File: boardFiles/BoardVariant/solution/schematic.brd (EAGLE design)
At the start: 75.9 x 38.1 mm, 45 parts, among them IC1 MSP430F1491, IC3 CP2102, U1 TPS62122_DRV_6

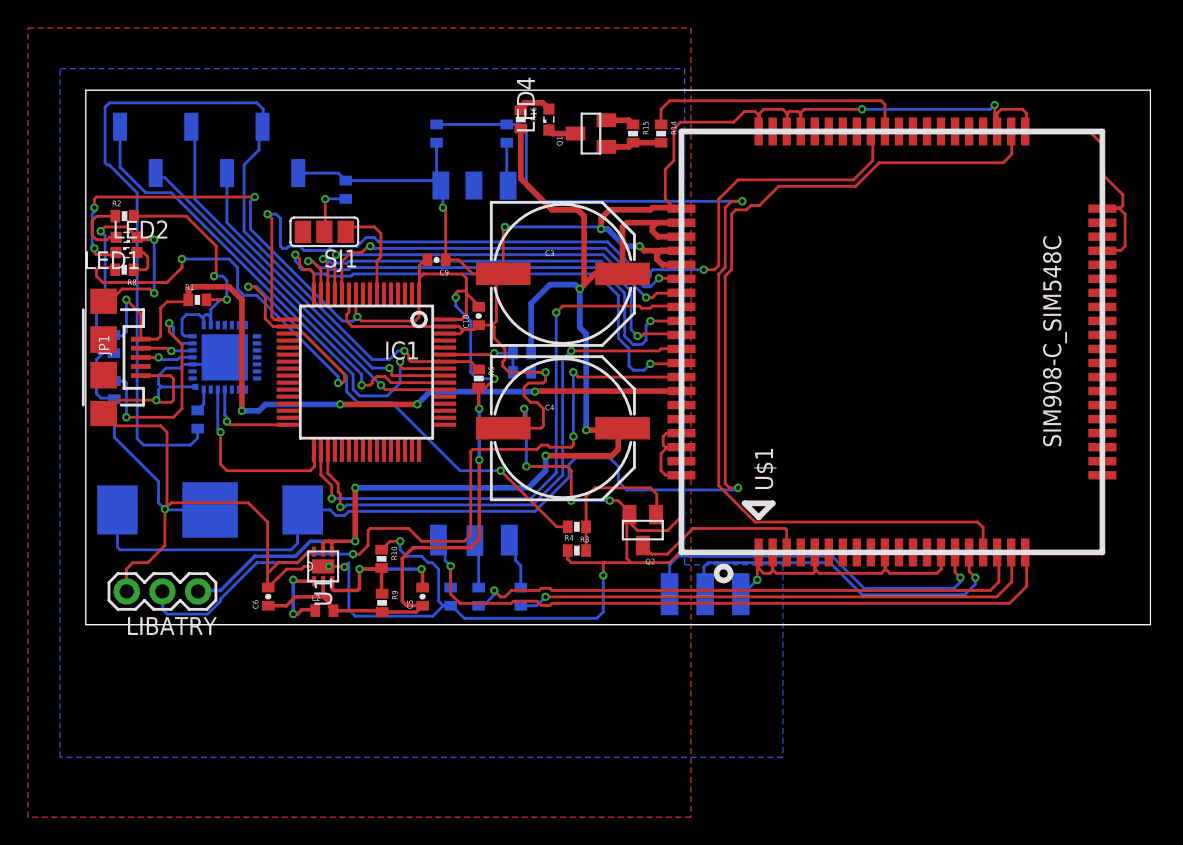
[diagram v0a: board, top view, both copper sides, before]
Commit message: normal push
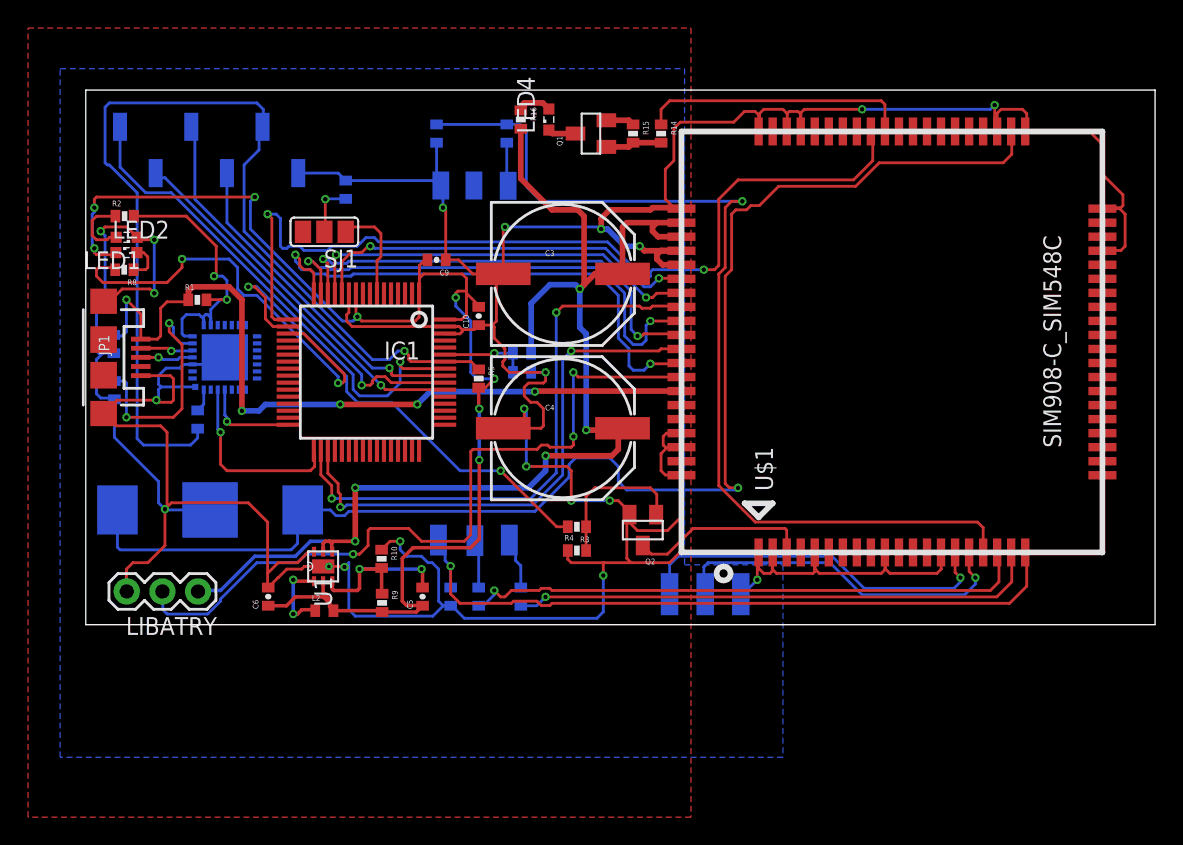
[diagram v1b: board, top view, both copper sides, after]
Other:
- board size 75.9 x 38.1 mm -> 76.2 x 38.1 mm
